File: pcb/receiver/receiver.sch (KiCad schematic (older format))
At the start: 37 parts, among them J101 Conn_01x02, Q101 BSS215PH6327XTSA1, Q102 MMBT2222A-7-F, U101 TPS63700DRCR, U102 NCP1403SNT1G

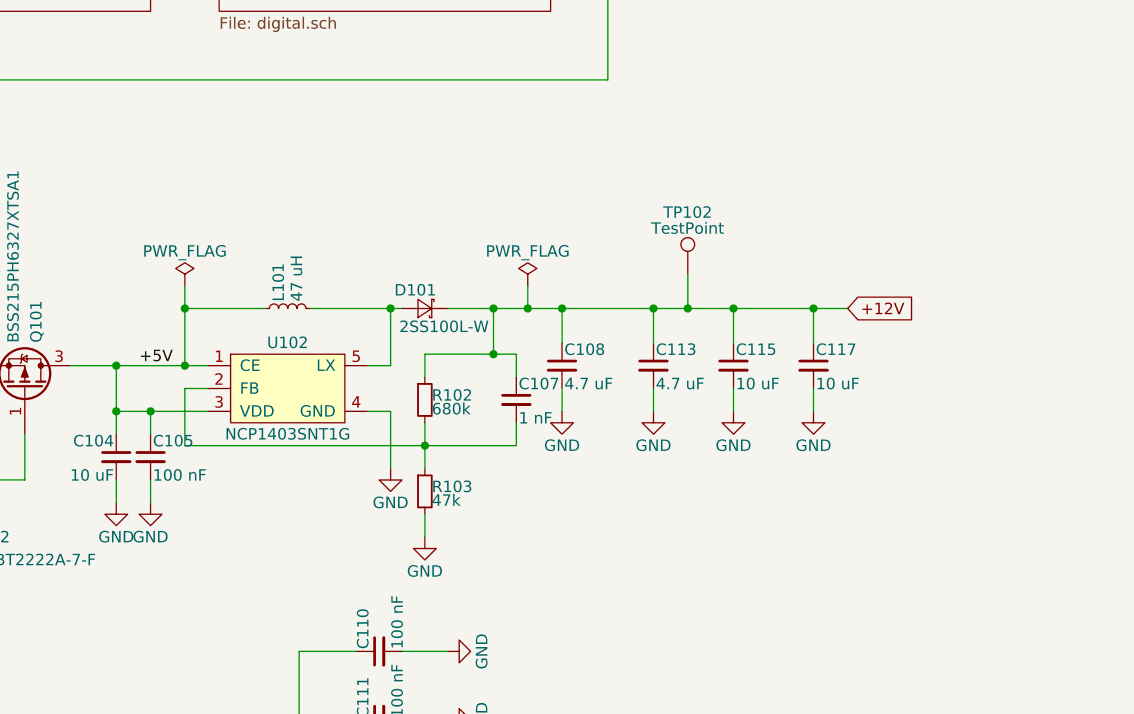
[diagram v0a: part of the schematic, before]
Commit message: I guess I modified some of the schematics somewhere?
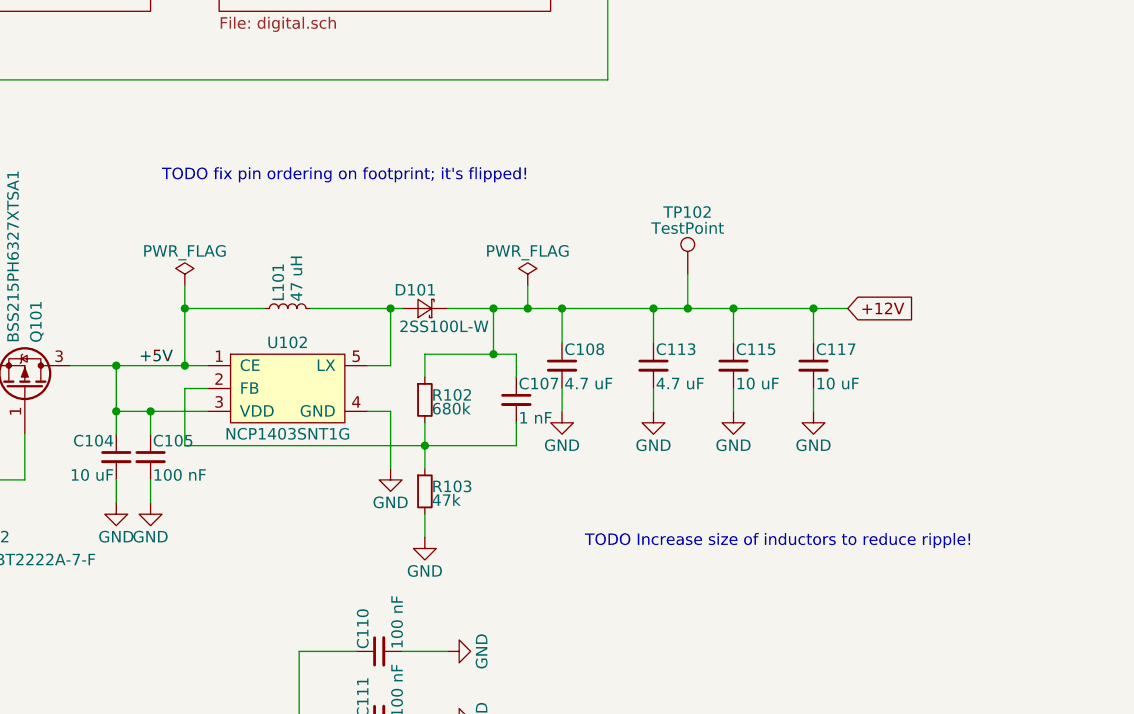
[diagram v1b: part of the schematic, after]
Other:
- note added: "TODO Increase size of inductors to reduce ripple!"
- note added: "TODO fix pin ordering on footprint; it's flipped!"
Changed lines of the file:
@@
 Wire Wire Line
 	4950 6700 4950 6800
+Text Notes 3250 3750 0    50   ~ 0
+TODO fix pin ordering on footprint; it's flipped!
+Text Notes 5100 5350 0    50   ~ 0
+TODO Increase size of inductors to reduce ripple!
 $EndSCHEMATC
